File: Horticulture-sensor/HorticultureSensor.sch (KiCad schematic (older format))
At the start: 24 parts, among them J1 Conn_01x04, J2 Conn_02x05_Odd_Even, J3 Conn_01x03, J4 Conn_01x04, J5 Conn_01x03, J6 Conn_01x02, J7 Conn_01x02, J8 Conn_01x02, Q1 IRLML2030TRPBF, Q2 IRLML2030TRPBF, U1 STM32F030F4Px, U2 ENS210, U3 MCP1700-3302E_TO

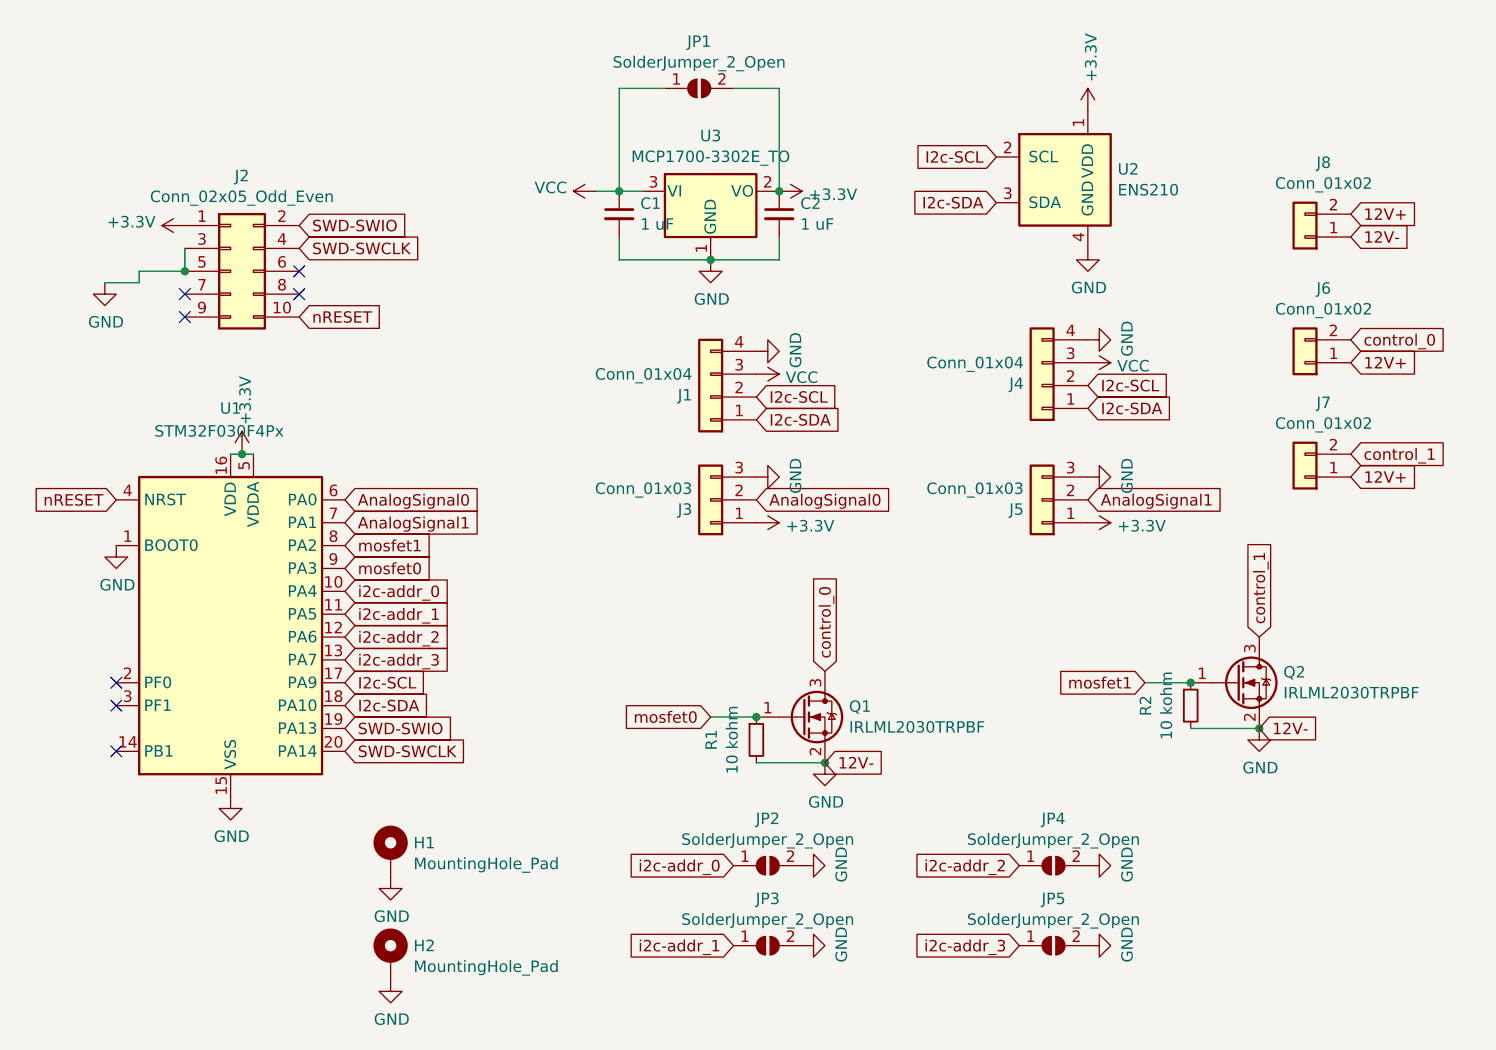
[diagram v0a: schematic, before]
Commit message: Resolves #4 #6 #5
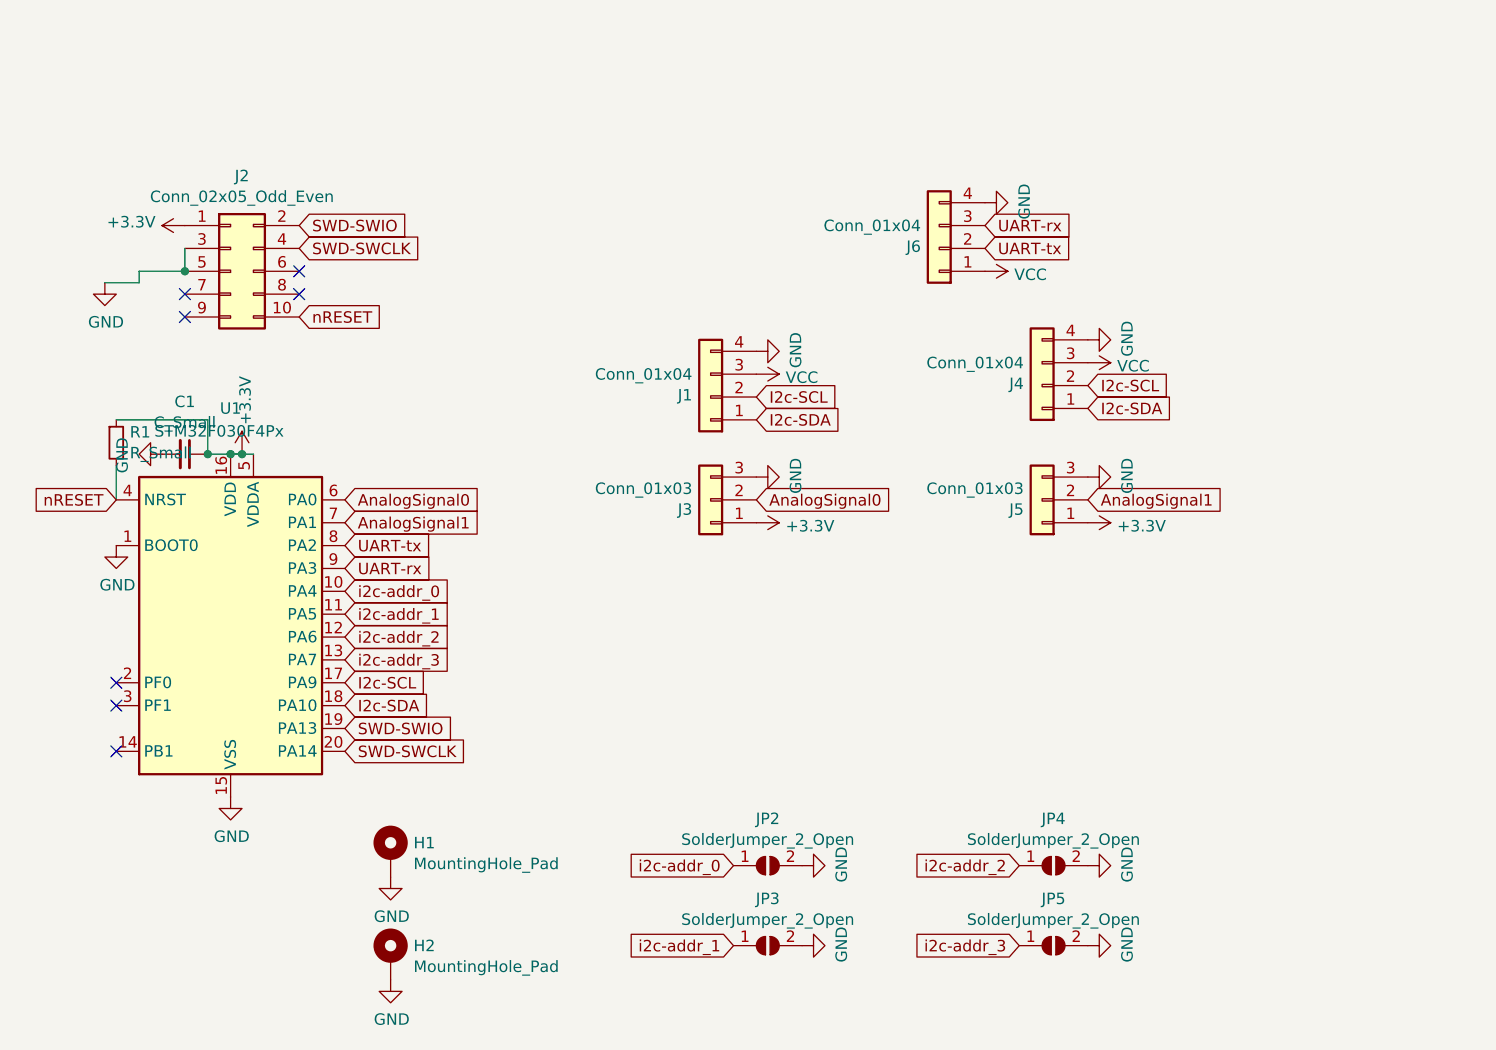
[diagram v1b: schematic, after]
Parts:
- removed C2: 1 uF, Capacitor_SMD:C_0805_2012Metric, symbol Device:C_Small
- removed J6, J7, J8: Conn_01x02, Connector_JST:JST_XH_B2B-XH-AM_1x02_P2.50mm_Vertical, symbol Connector_Generic:Conn_01x02
- removed JP1: SolderJumper_2_Open, Jumper:SolderJumper-2_P1.3mm_Open_RoundedPad1.0x1.5mm, symbol Jumper:SolderJumper_2_Open
- removed Q1, Q2: IRLML2030TRPBF, Package_TO_SOT_SMD:SOT-23, symbol Transistor_FET:IRLML0030
- removed R2: 10 kohm, Resistor_SMD:R_0805_2012Metric, symbol Device:R_Small
- removed U2: ENS210, Package_DFN_QFN:AMS_QFN-4-1EP_2x2mm_P0.95mm_EP0.7x1.6mm, symbol Sensor_Humidity:ENS210
- removed U3: MCP1700-3302E_TO, Package_TO_SOT_SMD:SOT-23, symbol Regulator_Linear:MCP1700-1202E_SOT23
- added J6: Conn_01x04, Connector_Molex:Molex_PicoBlade_53398-0471_1x04-1MP_P1.25mm_Vertical, symbol Connector_Generic:Conn_01x04
- C1: value 1 uF -> C_Small
- J1, J4: footprint Connector_JST:JST_XH_S4B-XH-A-1_1x04_P2.50mm_Horizontal -> Connector_Molex:Molex_PicoBlade_53398-0471_1x04-1MP_P1.25mm_Vertical
- J3, J5: footprint Connector_JST:JST_XH_B3B-XH-A_1x03_P2.50mm_Vertical -> Connector_Molex:Molex_PicoBlade_53398-0371_1x03-1MP_P1.25mm_Vertical
- R1: value 10 kohm -> R_Small
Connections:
- net +3V3: now also C1.1, R1.1
- net GND: now also J6.4 (Pin_4); no longer R1.2
- net VCC: now also J6.1 (Pin_1); no longer C1.1
- net nRESET: now also R1.2
- net mosfet0 renamed UART-rx
- net UART-rx: now also J6.3 (Pin_3); no longer R1.1
- net mosfet1 renamed UART-tx
- net UART-tx: now also J6.2 (Pin_2)

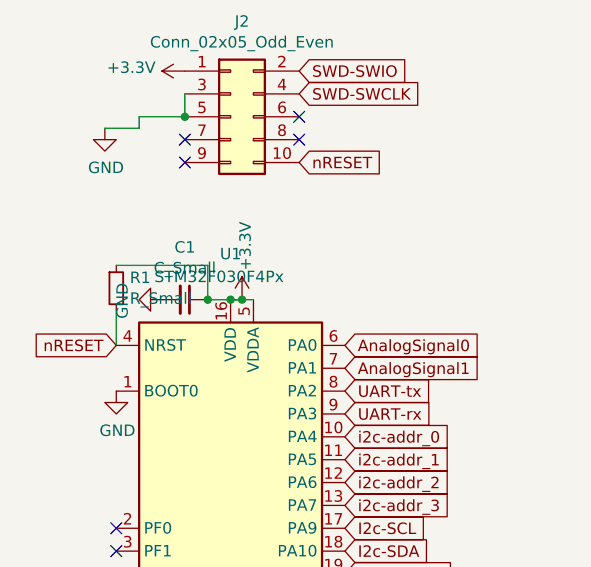
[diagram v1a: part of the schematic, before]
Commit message: Resolves #2
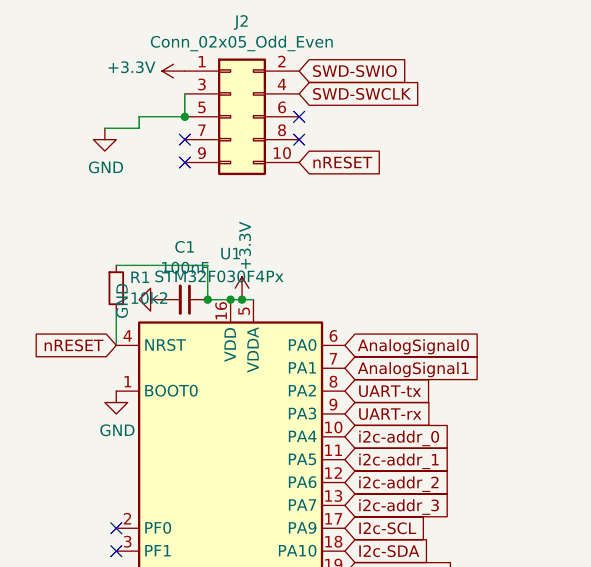
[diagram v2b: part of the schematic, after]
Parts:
- C1: value C_Small -> 100nF
- R1: value R_Small -> 10k2
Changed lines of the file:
@@
 P 7950 6950
 F 0 "C1" V 7721 6950 50  0000 C CNN
-F 1 "C_Small" V 7812 6950 50  0000 C CNN
+F 1 "100nF" V 7812 6950 50  0000 C CNN
 F 2 "Capacitor_SMD:C_0805_2012Metric" H 7950 6950 50  0001 C CNN
 F 3 "~" H 7950 6950 50  0001 C CNN
@@
 P 7650 6900
 F 0 "R1" H 7709 6946 50  0000 L CNN
-F 1 "R_Small" H 7709 6855 50  0000 L CNN
+F 1 "10k2" H 7709 6855 50  0000 L CNN
 F 2 "Resistor_SMD:R_0805_2012Metric" H 7650 6900 50  0001 C CNN
 F 3 "~" H 7650 6900 50  0001 C CNN
@@
 Connection ~ 8050 6950
 Connection ~ 8150 6950
-Wire Wire Line
-	8150 6950 8200 6950
 $Comp
 L power:GND #PWR0111
